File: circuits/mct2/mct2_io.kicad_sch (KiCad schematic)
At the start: 183 parts

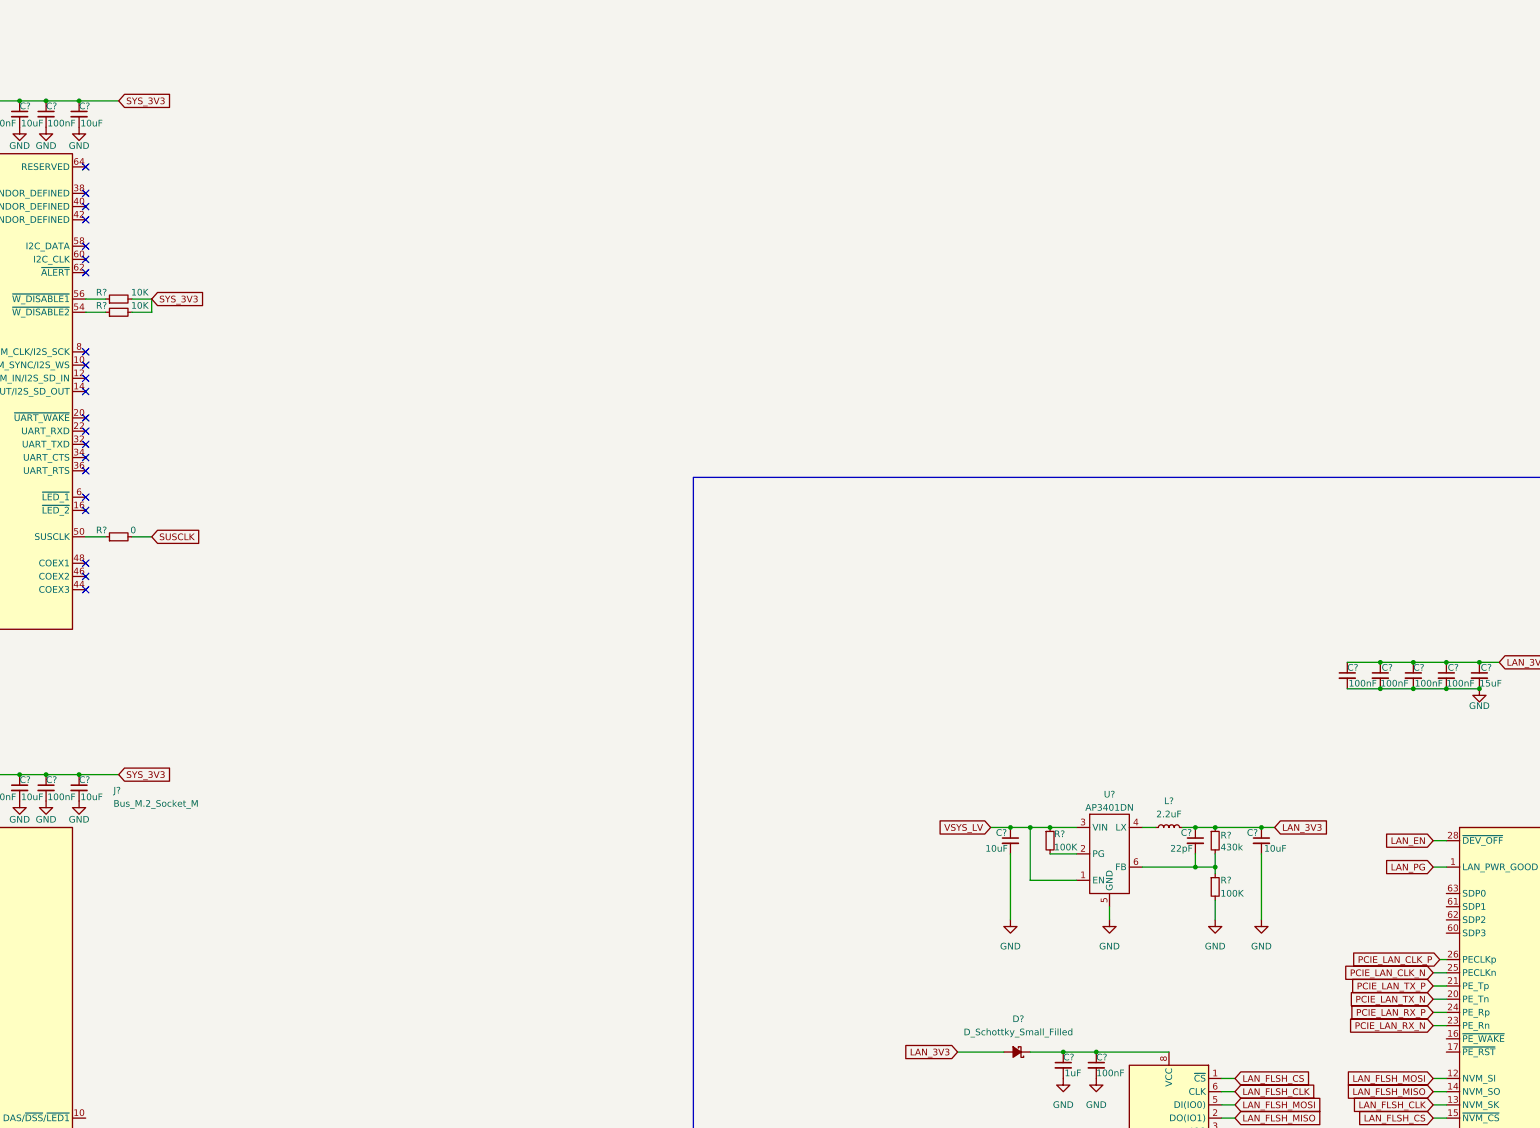
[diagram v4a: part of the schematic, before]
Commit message: Aug 17, 2024 2
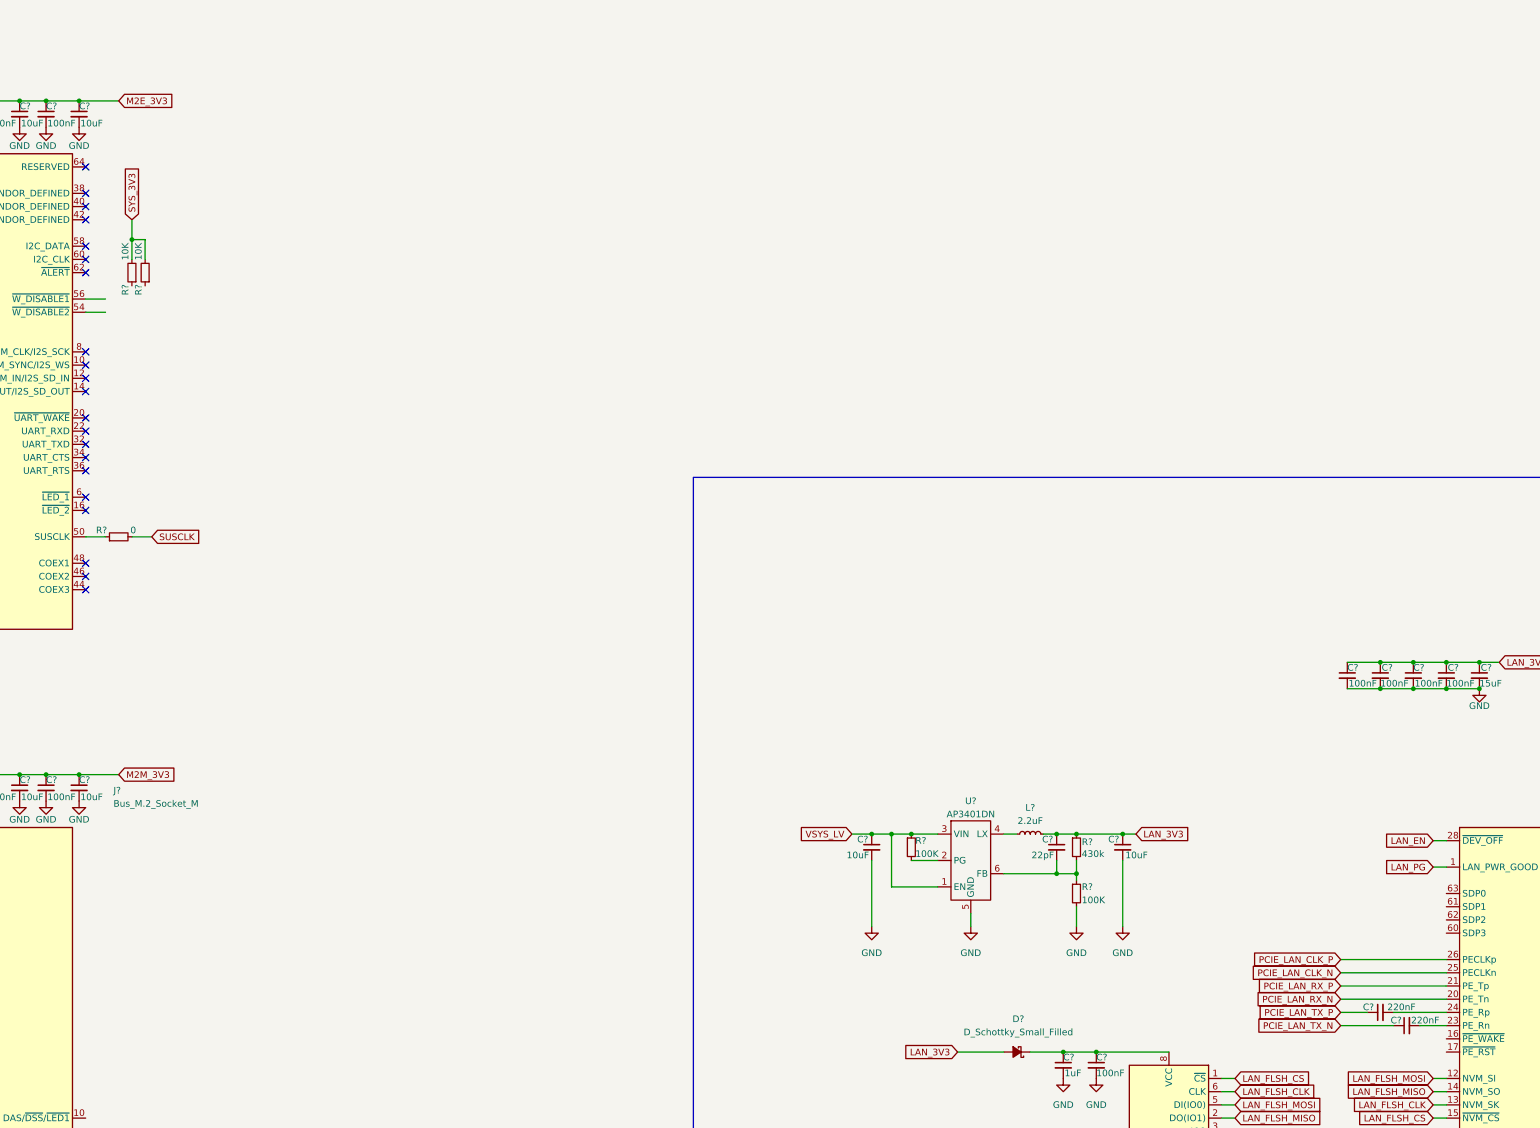
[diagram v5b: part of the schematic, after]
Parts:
- added C? (x2): 220nF, symbol Device:C_Small
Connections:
- net PCIE_LAN_RX_N: now also U?.20 (PE_Tn); no longer U?.23 (PE_Rn)
- net PCIE_LAN_RX_P: now also U?.21 (PE_Tp); no longer U?.24 (PE_Rp)
- net PCIE_LAN_TX_N: now also C?.1; no longer U?.20 (PE_Tn)
- net PCIE_LAN_TX_P: now also C?.1; no longer U?.21 (PE_Tp)
- net SYS_3V3: no longer C?.1, C?.1, C?.1, C?.1, C?.1, C?.1, C?.1, C?.1, J?.12 (3.3V), J?.14 (3.3V), J?.16 (3.3V), J?.18 (3.3V), J?.2 (3.3V), J?.2 (3.3V), J?.4 (3.3V), J?.4 (3.3V), J?.70 (3.3V), J?.72 (3.3V), J?.72 (3.3V), J?.74 (3.3V), J?.74 (3.3V)
- net at R?.1: no longer J?.54 (~{W_DISABLE2})
- net at R?.1: no longer J?.56 (~{W_DISABLE1})
- new net: C?.2, U?.23 (PE_Rn)
- new net: C?.2, U?.24 (PE_Rp)
- new net M2E_3V3: C?.1, C?.1, C?.1, C?.1, J?.2 (3.3V), J?.4 (3.3V), J?.72 (3.3V), J?.74 (3.3V)
- new net M2M_3V3: C?.1, C?.1, C?.1, C?.1, J?.12 (3.3V), J?.14 (3.3V), J?.16 (3.3V), J?.18 (3.3V), J?.2 (3.3V), J?.4 (3.3V), J?.70 (3.3V), J?.72 (3.3V), J?.74 (3.3V)
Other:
- moved on the sheet: C?, L?, R?, U?
